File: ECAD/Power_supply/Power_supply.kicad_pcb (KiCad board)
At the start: 2 copper layers, 40 parts, among them J1 Barrel_Jack_Switch, J2 Conn_01x06, Q1 DMP3037LSS-13, SW1 SW_Push_DPDT, U1 LM317_TO-220, U2 LM317_TO-220

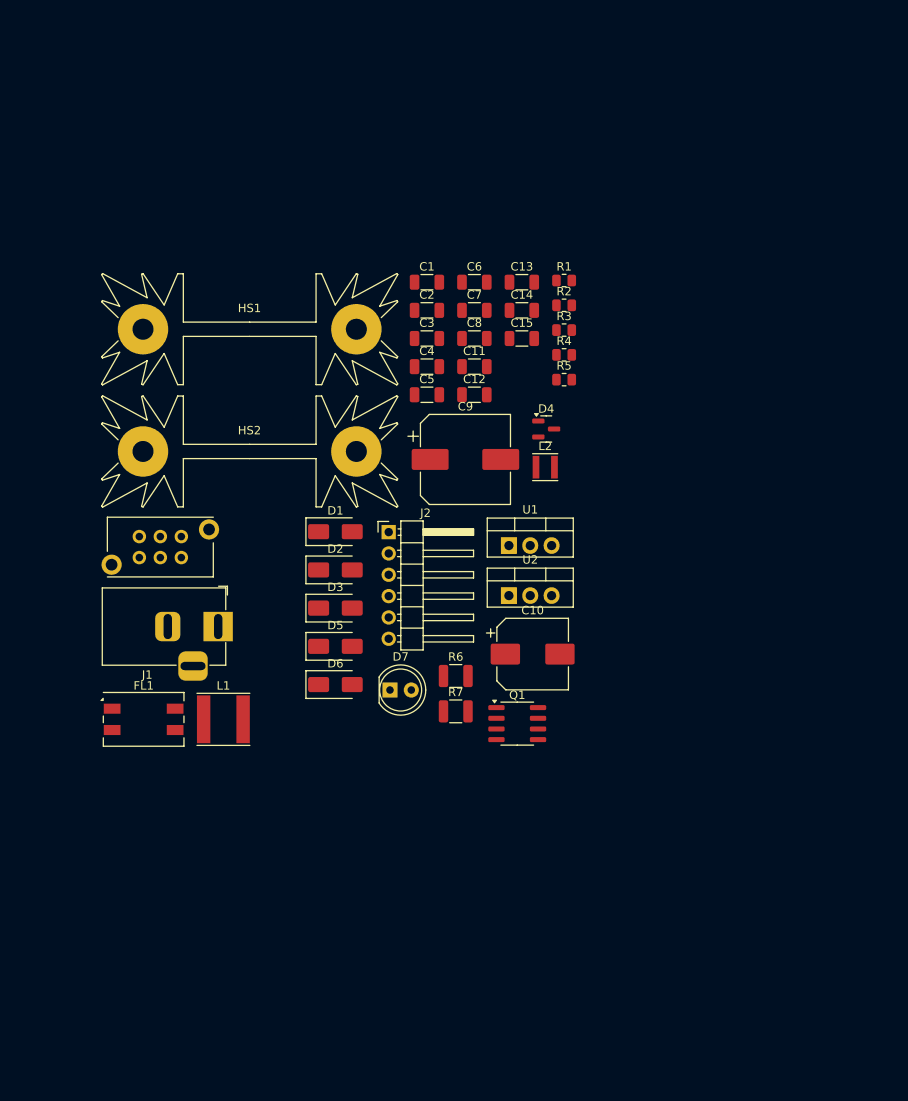
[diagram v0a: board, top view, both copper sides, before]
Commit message: Progressed PCB layout.
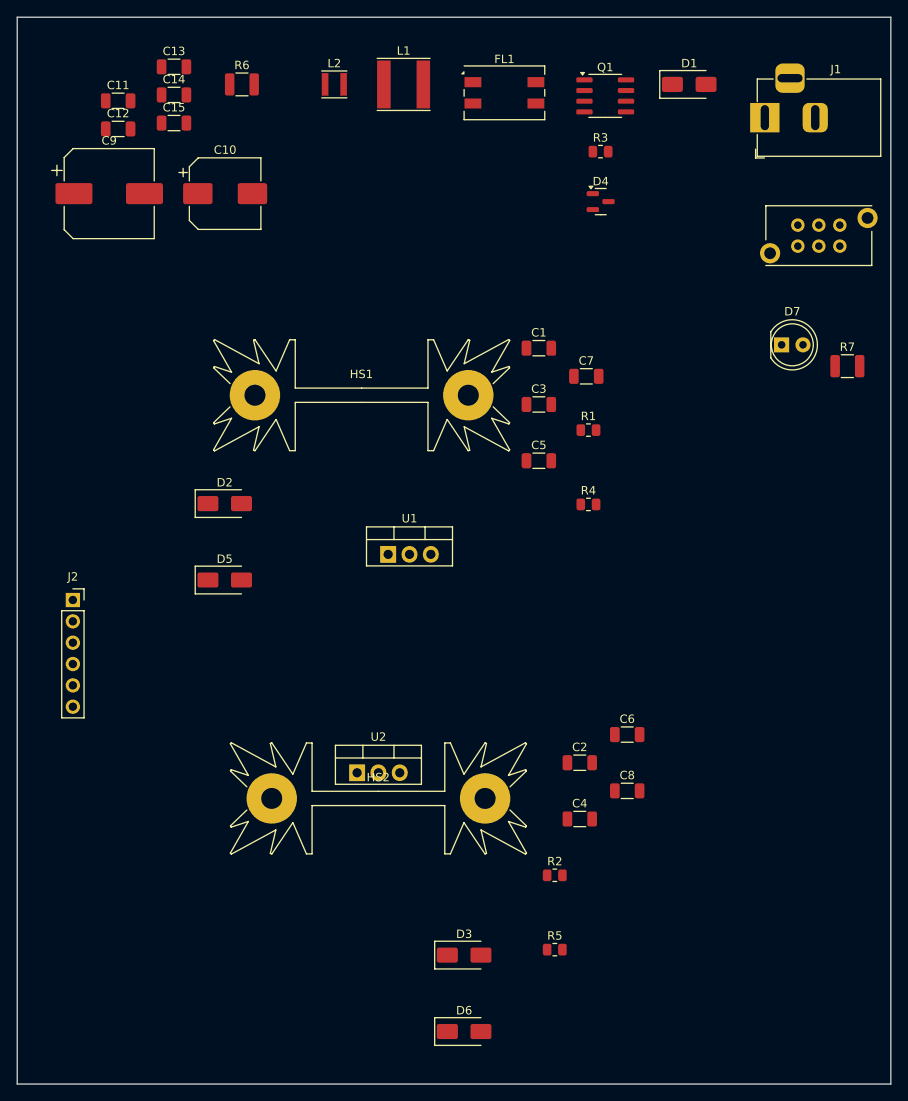
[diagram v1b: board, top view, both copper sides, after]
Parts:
- J2: footprint Connector_PinHeader_2.54mm:PinHeader_1x06_P2.54mm_Horizontal -> Connector_PinSocket_2.54mm:PinSocket_1x06_P2.54mm_Vertical
- moved J1 88.9 mm to (180.0, 48.0), turned to 180 degrees
- moved SW1 86.7 mm to (186.4, 62.0)
- moved FL1 86.1 mm to (149.0, 45.0)
- moved L1 78.6 mm to (137.0, 44.0)
- moved Q1 75.5 mm to (161.0, 45.4)
- moved R6 74.9 mm to (117.8, 44.0)
- moved D1 67.9 mm to (171.0, 44.0)
- moved R2 67.9 mm to (155.0, 138.2)
- moved R5 67.9 mm to (155.0, 147.0)
- moved C10 65.9 mm to (115.8, 57.0)
- moved D7 62.2 mm to (182.0, 75.0)
- moved R7 62.2 mm to (189.8, 77.5)
- moved C2 56.8 mm to (158.0, 124.8)
- moved C6 56.8 mm to (163.6, 121.4)
- moved C4 56.8 mm to (158.0, 131.4)
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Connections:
- J2 pad 1: +12V -> +5V
- J2 pad 3: +9V -> +12V
- J2 pad 5: +5V -> +9V
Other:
- board outline added: 104 x 127 mm
